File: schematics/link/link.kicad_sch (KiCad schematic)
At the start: 21 parts, among them J1 S2, J10 TC, J2 ARJM11C7-114-BA-EW2, J3 SDI12, J4 S1

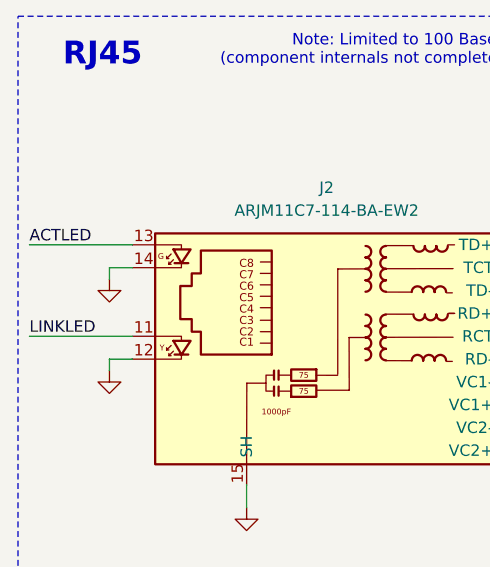
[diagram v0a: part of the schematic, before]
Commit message: GPT review pt2
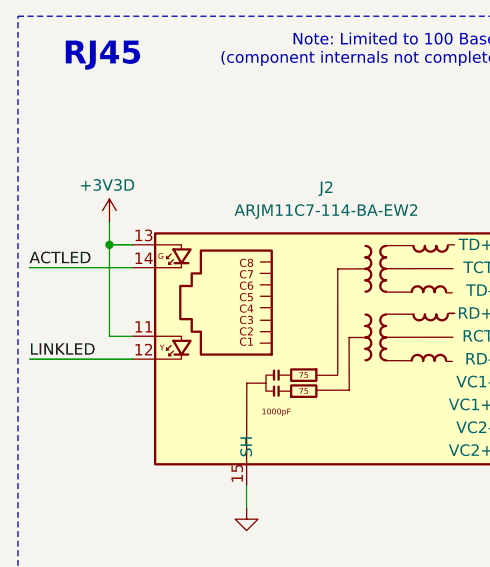
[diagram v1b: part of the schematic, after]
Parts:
- R3: MPN RC0402FR-0710RL -> RT0402BRD0710RL
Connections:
- net ACTLED: now also J2.14; no longer J2.13
- net GND: no longer J2.12, J2.14
- net LINKLED: now also J2.12; no longer J2.11
- new net +3V3D: J2.11, J2.13
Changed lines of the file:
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@@
 	)
 	(junction
+		(at 35.56 114.3)
+		(diameter 0)
+		(color 0 0 0 0)
+	)
+	(junction
 		(at 96.52 166.37)
 		(diameter 0)
@@
 	(wire
 		(pts
-			(xy 129.54 49.53) (xy 134.62 49.53)
+			(xy 35.56 111.76) (xy 35.56 114.3)
 		)
 		(stroke
@@
 	(wire
 		(pts
-			(xy 35.56 116.84) (xy 35.56 118.11)
+			(xy 129.54 49.53) (xy 134.62 49.53)
 		)
 		(stroke
@@
 	(wire
 		(pts
-			(xy 38.1 127) (xy 35.56 127)
-		)
-		(stroke
-			(width 0)
-			(type default)
-		)
-	)
-	(wire
-		(pts
 			(xy 153.67 137.16) (xy 154.94 137.16)
 		)
@@
 	(wire
 		(pts
-			(xy 252.73 52.07) (xy 261.62 52.07)
+			(xy 35.56 114.3) (xy 35.56 124.46)
 		)
 		(stroke
@@
 	(wire
 		(pts
-			(xy 81.28 119.38) (xy 106.68 119.38)
+			(xy 252.73 52.07) (xy 261.62 52.07)
 		)
 		(stroke
@@
 	(wire
 		(pts
-			(xy 26.67 114.3) (xy 38.1 114.3)
+			(xy 81.28 119.38) (xy 106.68 119.38)
 		)
 		(stroke
@@
 	(wire
 		(pts
-			(xy 35.56 116.84) (xy 38.1 116.84)
-		)
-		(stroke
-			(width 0)
-			(type default)
-		)
-	)
-	(wire
-		(pts
 			(xy 246.38 114.3) (xy 246.38 128.27)
 		)
@@
 	(wire
 		(pts
+			(xy 26.67 116.84) (xy 38.1 116.84)
+		)
+		(stroke
+			(width 0)
+			(type default)
+		)
+	)
+	(wire
+		(pts
 			(xy 148.59 130.81) (xy 148.59 134.62)
 		)
@@
 	(wire
 		(pts
-			(xy 26.67 124.46) (xy 38.1 124.46)
+			(xy 26.67 127) (xy 38.1 127)
 		)
 		(stroke
@@
 	(wire
 		(pts
-			(xy 35.56 127) (xy 35.56 128.27)
+			(xy 153.67 132.08) (xy 153.67 130.81)
 		)
 		(stroke
@@
 	(wire
 		(pts
-			(xy 153.67 132.08) (xy 153.67 130.81)
+			(xy 246.38 128.27) (xy 246.38 142.24)
 		)
 		(stroke
@@
 	(wire
 		(pts
-			(xy 246.38 128.27) (xy 246.38 142.24)
+			(xy 259.08 147.32) (xy 257.81 147.32)
 		)
 		(stroke
@@
 	(wire
 		(pts
-			(xy 259.08 147.32) (xy 257.81 147.32)
+			(xy 148.59 109.22) (xy 148.59 113.03)
 		)
 		(stroke
@@
 	(wire
 		(pts
-			(xy 148.59 109.22) (xy 148.59 113.03)
+			(xy 81.28 116.84) (xy 119.38 116.84)
 		)
 		(stroke
@@
 	(wire
 		(pts
-			(xy 81.28 116.84) (xy 119.38 116.84)
+			(xy 80.01 147.32) (xy 86.36 147.32)
 		)
 		(stroke
@@
 	(wire
 		(pts
-			(xy 80.01 147.32) (xy 86.36 147.32)
+			(xy 38.1 124.46) (xy 35.56 124.46)
 		)
 		(stroke
@@
 	(wire
 		(pts
+			(xy 38.1 114.3) (xy 35.56 114.3)
+		)
+		(stroke
+			(width 0)
+			(type default)
+		)
+	)
+	(wire
+		(pts
 			(xy 227.33 110.49) (xy 228.6 110.49)
 		)
@@
 	)
 	(label "LINKLED"
-		(at 26.67 124.46 0)
+		(at 26.67 127 0)
 		(effects
 			(font
@@
 	)
 	(label "ACTLED"
-		(at 26.67 114.3 0)
+		(at 26.67 116.84 0)
 		(effects
 			(font
@@
 	)
 	(symbol
-		(lib_id "power:GND")
-		(at 35.56 118.11 0)
-		(mirror y)
-		(unit 1)
-		(body_style 1)
-		(exclude_from_sim no)
-		(in_bom yes)
-		(on_board yes)
-		(in_pos_files yes)
-		(dnp no)
-		(property "Reference" "#PWR03"
-			(at 35.56 124.46 0)
-			(hide yes)
-			(show_name no)
-			(do_not_autoplace no)
-			(effects
-				(font
-					(size 1.27 1.27)
-				)
-			)
-		)
-		(property "Value" "GND"
-			(at 31.496 119.888 0)
-			(hide yes)
-			(show_name no)
-			(do_not_autoplace no)
-			(effects
-				(font
-					(size 1.27 1.27)
-				)
-			)
-		)
-		(property "Footprint" ""
-			(at 35.56 118.11 0)
-			(hide yes)
-			(show_name no)
-			(do_not_autoplace no)
-			(effects
-				(font
-					(size 1.27 1.27)
-				)
-			)
-		)
-		(property "Datasheet" ""
-			(at 35.56 118.11 0)
-			(hide yes)
-			(show_name no)
-			(do_not_autoplace no)
-			(effects
-				(font
-					(size 1.27 1.27)
-				)
-			)
-		)
-		(property "Description" "Power symbol creates a global label with name \"GND\" , ground"
-			(at 35.56 118.11 0)
-			(hide yes)
-			(show_name no)
-			(do_not_autoplace no)
-			(effects
-				(font
-					(size 1.27 1.27)
-				)
-			)
-		)
-		(pin "1"
-		)
-		(instances
-			(project "link"
-				(path "/e6a73b1b-9233-47b9-8d6b-253608bed688"
-					(reference "#PWR03")
-					(unit 1)
-				)
-			)
-		)
-	)
-	(symbol
 		(lib_id "power:+12V")
 		(at 148.59 130.81 0)
@@
 			)
 		)
-		(property "MPN" "RC0402FR-0710RL"
+		(property "MPN" "RT0402BRD0710RL"
 			(at 119.38 111.76 0)
 			(hide yes)
@@
 	(symbol
 		(lib_id "power:GND")
-		(at 35.56 128.27 0)
-		(mirror y)
-		(unit 1)
-		(body_style 1)
-		(exclude_from_sim no)
-		(in_bom yes)
-		(on_board yes)
-		(in_pos_files yes)
-		(dnp no)
-		(property "Reference" "#PWR010"
-			(at 35.56 134.62 0)
-			(hide yes)
-			(show_name no)
-			(do_not_autoplace no)
-			(effects
-				(font
-					(size 1.27 1.27)
-				)
-			)
-		)
-		(property "Value" "GND"
-			(at 31.496 130.048 0)
-			(hide yes)
-			(show_name no)
-			(do_not_autoplace no)
-			(effects
-				(font
-					(size 1.27 1.27)
-				)
-			)
-		)
-		(property "Footprint" ""
-			(at 35.56 128.27 0)
-			(hide yes)
-			(show_name no)
-			(do_not_autoplace no)
-			(effects
-				(font
-					(size 1.27 1.27)
-				)
-			)
-		)
-		(property "Datasheet" ""
-			(at 35.56 128.27 0)
-			(hide yes)
-			(show_name no)
-			(do_not_autoplace no)
-			(effects
-				(font
-					(size 1.27 1.27)
-				)
-			)
-		)
-		(property "Description" "Power symbol creates a global label with name \"GND\" , ground"
-			(at 35.56 128.27 0)
-			(hide yes)
-			(show_name no)
-			(do_not_autoplace no)
-			(effects
-				(font
-					(size 1.27 1.27)
-				)
-			)
-		)
-		(pin "1"
-		)
-		(instances
-			(project "link"
-				(path "/e6a73b1b-9233-47b9-8d6b-253608bed688"
-					(reference "#PWR010")
-					(unit 1)
-				)
-			)
-		)
-	)
-	(symbol
-		(lib_id "power:GND")
 		(at 153.67 116.84 0)
 		(mirror y)
@@
 					(unit 1)
 				)
+			)
+		)
+	)
+	(symbol
+		(lib_id "power:+3V3")
+		(at 35.56 111.76 0)
+		(unit 1)
+		(body_style 1)
+		(exclude_from_sim no)
+		(in_bom yes)
+		(on_board yes)
+		(in_pos_files yes)
+		(dnp no)
+		(property "Reference" "#PWR0105"
+			(at 35.56 115.57 0)
+			(hide yes)
+			(show_name no)
+			(do_not_autoplace no)
+			(effects
+				(font
+					(size 1.27 1.27)
+				)
+			)
+		)
+		(property "Value" "+3V3D"
+			(at 35.306 107.696 0)
+			(show_name no)
+			(do_not_autoplace no)
+			(effects
+				(font
+					(size 1.27 1.27)
+				)
+			)
+		)
+		(property "Footprint" ""
+			(at 35.56 111.76 0)
+			(hide yes)
+			(show_name no)
+			(do_not_autoplace no)
+			(effects
+				(font
+					(size 1.27 1.27)
+				)
+			)
+		)
+		(property "Datasheet" ""
+			(at 35.56 111.76 0)
+			(hide yes)
+			(show_name no)
+			(do_not_autoplace no)
+			(effects
+				(font
+					(size 1.27 1.27)
+				)
+			)
+		)
+		(property "Description" "Power symbol creates a global label with name \"+3V3\""
+			(at 35.56 111.76 0)
+			(hide yes)
+			(show_name no)
+			(do_not_autoplace no)
+			(effects
+				(font
+					(size 1.27 1.27)
+				)
+			)
+		)
+		(pin "1"
+		)
+		(instances
+			(project "link"
+				(path "/e6a73b1b-9233-47b9-8d6b-253608bed688"
+					(reference "#PWR0105")
+					(unit 1)
+				)
